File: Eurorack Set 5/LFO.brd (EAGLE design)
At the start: 39.3 x 106.5 mm, 118 parts, among them IC1 LD1117AS33TR, IC3 TL074D, IC4 MCP6004, J1 PJ-341, J12 PJ-341, J13 PJ-341, J14 POWER, J2 PJ-341, J3 PJ-341, J4 PJ-341, J5 PJ-341, J6 PJ-341, J7 PJ-341, Q1 MMBT3904, Q3 MMBT3904, Q5 MMBT3904, U1 MKL02Z32VFK4, U2 LM4040DIM3-5.0, U4 74HC595BQ, U5 74HC595BQ, U6 24LC16T-I/OT, U7 MCP4822-E/SN

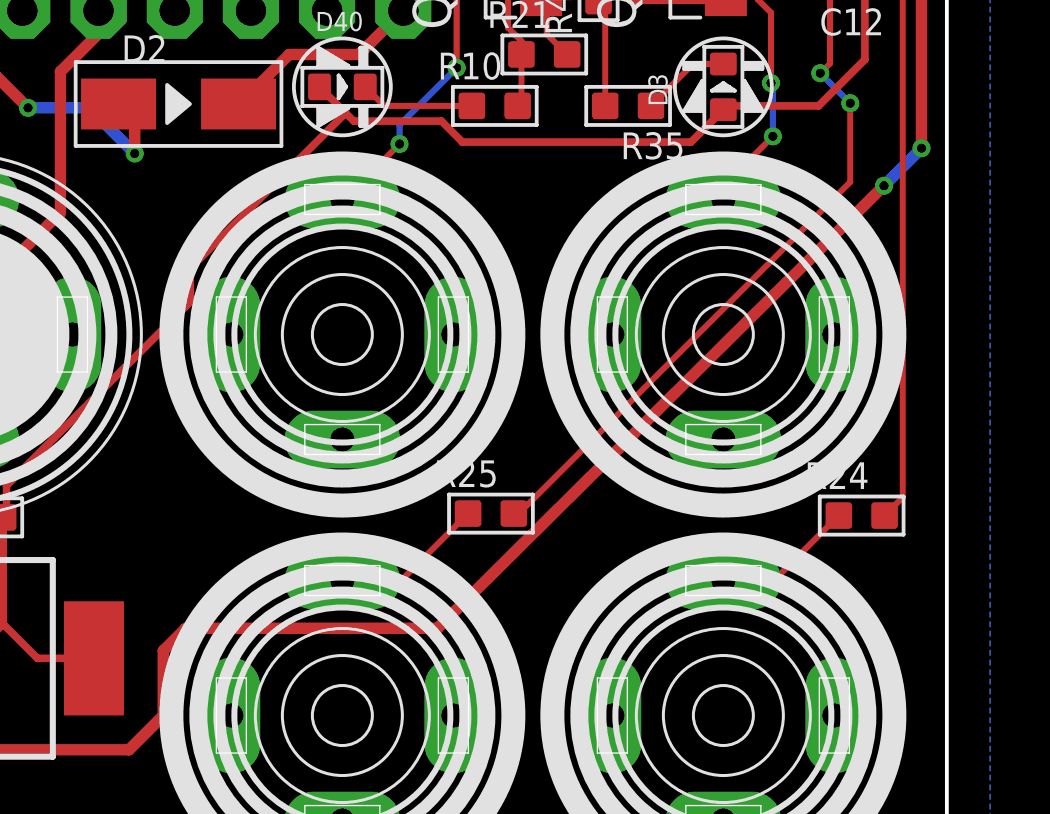
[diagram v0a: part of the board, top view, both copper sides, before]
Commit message: Doublechecks & artwork prep
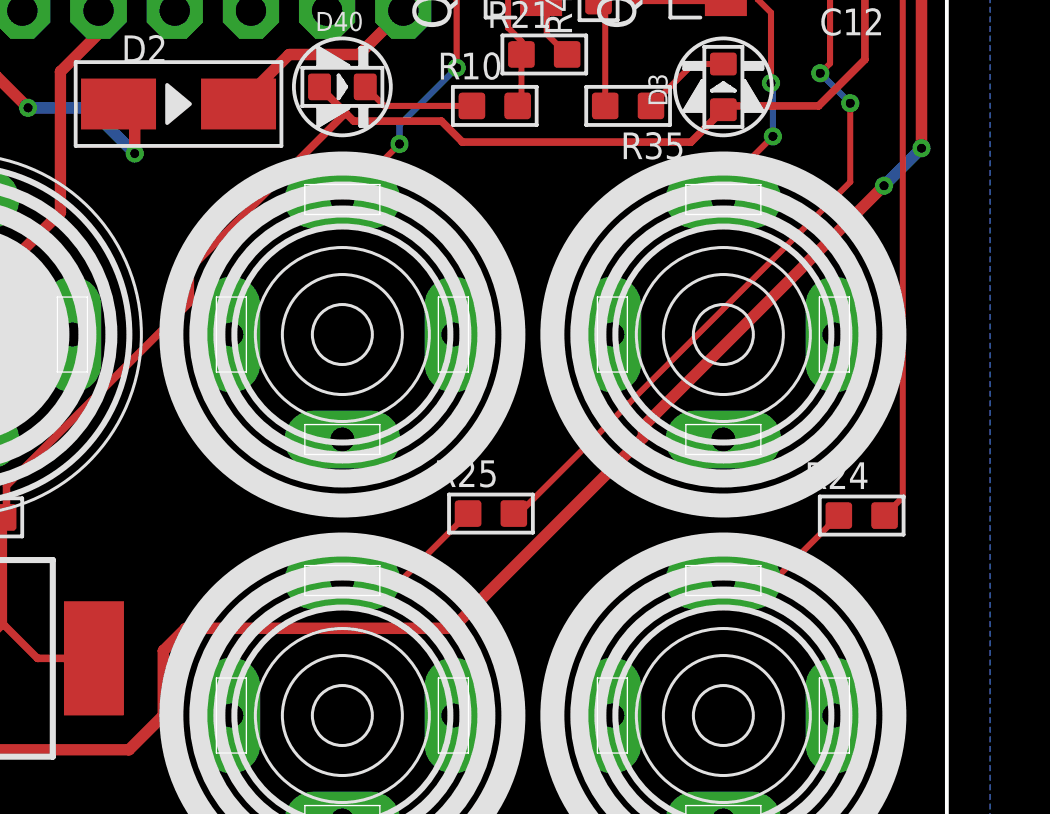
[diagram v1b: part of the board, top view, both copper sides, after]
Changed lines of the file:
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@@
 <?xml version="1.0" encoding="utf-8"?>
 <!DOCTYPE eagle SYSTEM "eagle.dtd">
-<eagle version="6.5.0">
+<eagle version="7.7.0">
 <drawing>
 <settings>
@@
 <pass name="Default">
 <param name="RoutingGrid" value="4.92125984mil"/>
+<param name="AutoGrid" value="1"/>
+<param name="Efforts" value="0"/>
+<param name="TopRouterVariant" value="1"/>
 <param name="tpViaShape" value="round"/>
 <param name="PrefDir.1" value="*"/>
@@
 <contactref element="IC4" pad="4"/>
 <contactref element="C17" pad="1"/>
-<contactref element="C17" pad="1"/>
 <contactref element="R29" pad="1"/>
 <contactref element="R17" pad="P$3"/>
@@
 <wire x1="5.588" y1="3.175" x2="5.08" y2="2.667" width="0.381" layer="1"/>
 <wire x1="5.08" y1="2.667" x2="5.08" y2="1.27" width="0.381" layer="1"/>
-<wire x1="23.494003125" y1="8.621003125" x2="15.098003125" y2="8.621003125" width="0.381" layer="1"/>
-<wire x1="38.375003125" y1="23.375003125" x2="23.494003125" y2="8.621003125" width="0.381" layer="1"/>
+<wire x1="23.988003125" y1="8.621003125" x2="15.098003125" y2="8.621003125" width="0.381" layer="1"/>
 <wire x1="39.625003125" y1="24.625003125" x2="38.375003125" y2="23.375003125" width="0.381" layer="16"/>
 <wire x1="39.625003125" y1="33.375003125" x2="39.625003125" y2="24.625003125" width="0.381" layer="1"/>
@@
 <wire x1="13.208" y1="4.572" x2="6.488" y2="4.572" width="0.381" layer="1"/>
 <wire x1="6.488" y1="4.572" x2="5.74" y2="5.32" width="0.381" layer="1"/>
+<wire x1="23.988003125" y1="8.621003125" x2="30.353" y2="14.986" width="0.381" layer="1"/>
+<wire x1="30.353" y1="14.986" x2="30.353" y2="15.353" width="0.381" layer="1"/>
+<wire x1="30.353" y1="15.353" x2="38.375003125" y2="23.375003125" width="0.381" layer="1"/>
 </signal>
 <signal name="N$25">
